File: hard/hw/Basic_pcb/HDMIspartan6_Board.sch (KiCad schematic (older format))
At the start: 50 parts

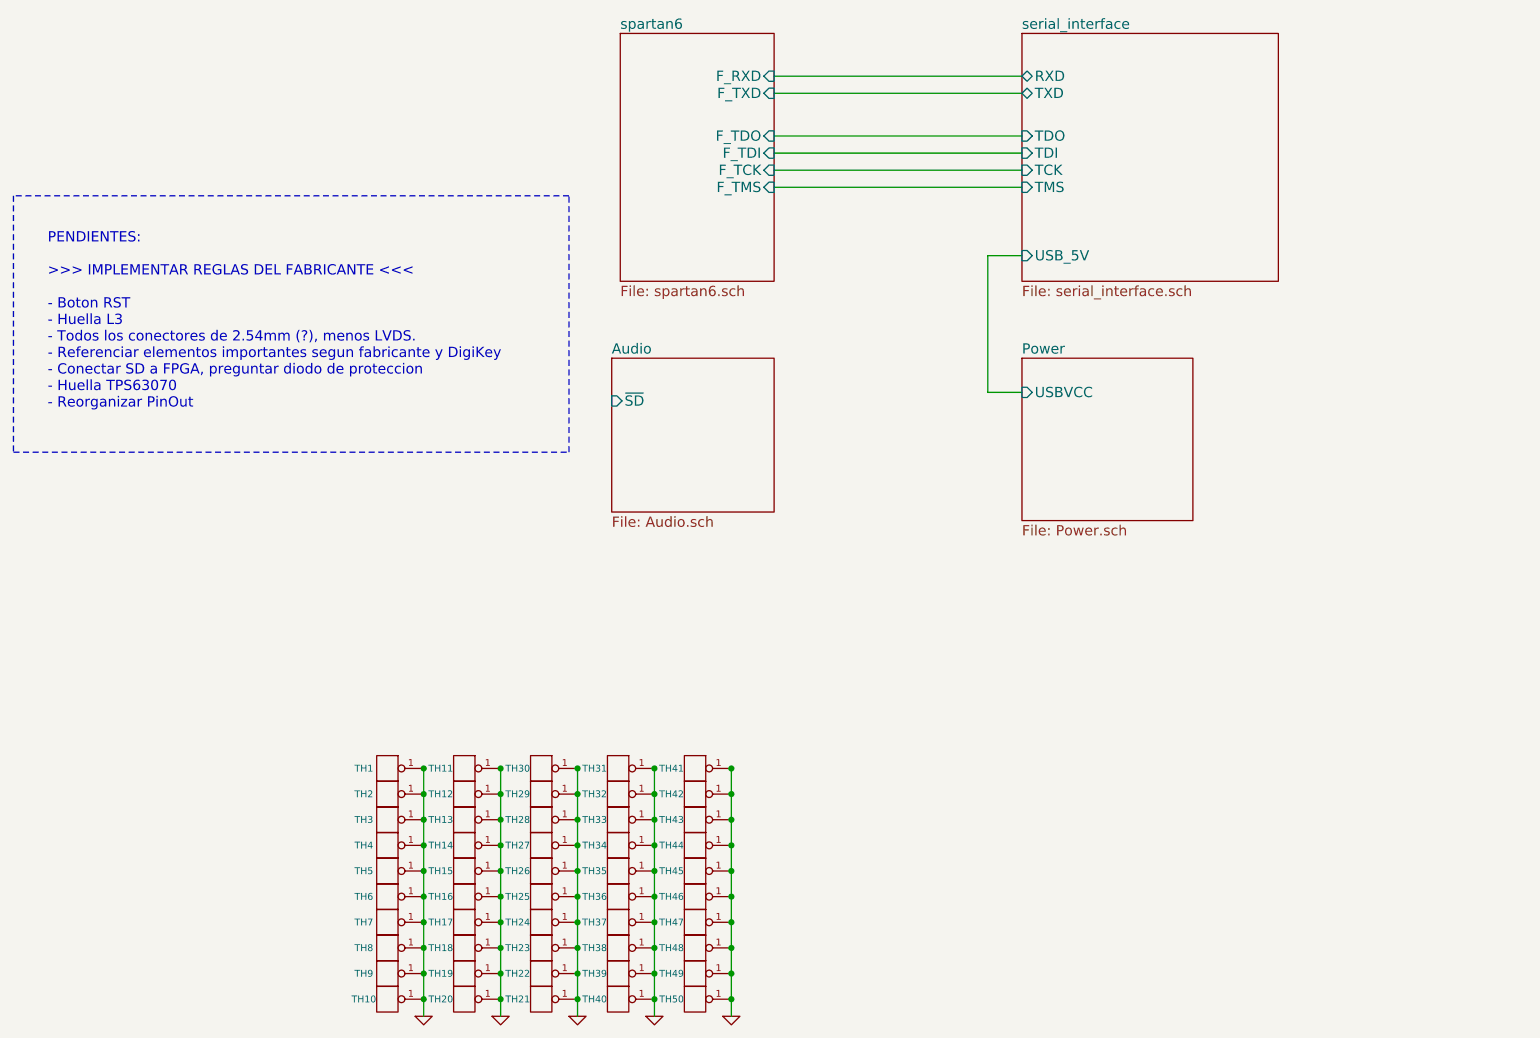
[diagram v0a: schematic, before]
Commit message: todas las huellas
by Ruben
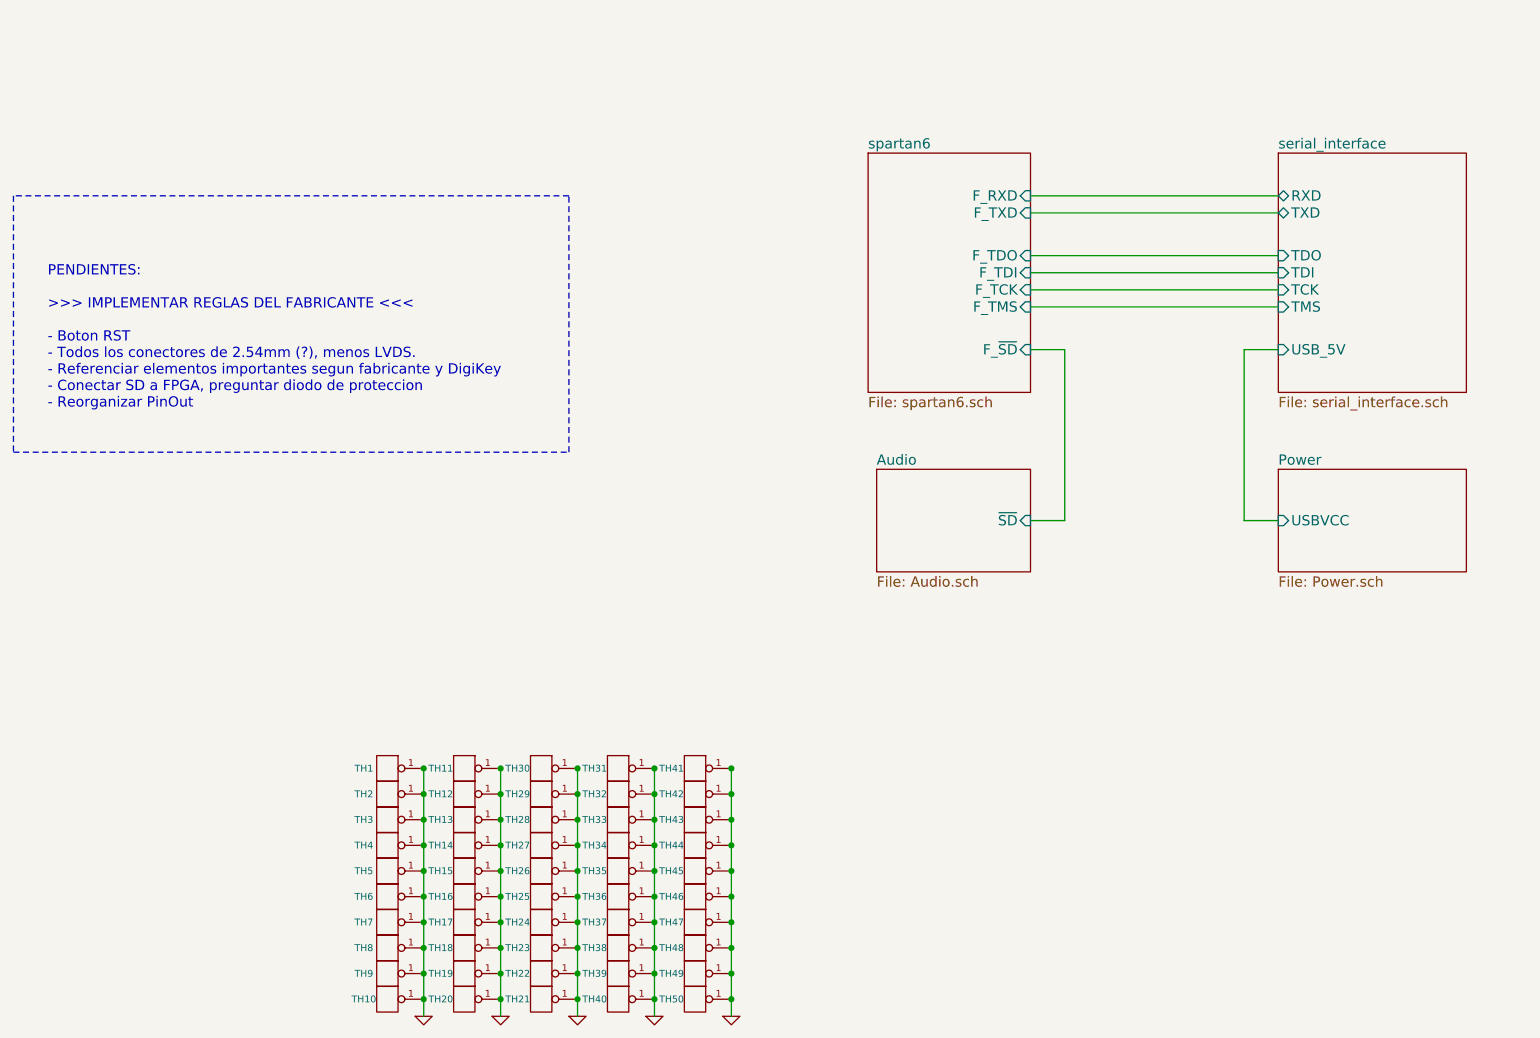
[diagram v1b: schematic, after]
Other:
- note added: "PENDIENTES:\n\n>>> IMPLEMENTAR REGLAS DEL FABRICANTE <<<\n\n- Boton RST\n- Todos los conectores de 2.54mm (?), menos LVDS.\n- Referenciar elementos importantes segun fabricante y DigiKey\n- Conectar SD a FPGA, preguntar diodo de proteccion\n- Reorganizar PinOut"
- note removed: "PENDIENTES:\n\n>>> IMPLEMENTAR REGLAS DEL FABRICANTE <<<\n\n- Boton RST\n- Huella L3\n- Todos los conectores de 2.54mm (?), menos LVDS.\n- Referenciar elementos importantes segun fabricante y DigiKey\n- Conectar SD a FPGA, preguntar diodo de proteccion\n- Huella TPS63070\n- Reorganizar PinOut"
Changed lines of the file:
@@
 $EndDescr
 $Sheet
-S 6650 1250 1500 1450
+S 8150 1950 1100 1400
 U 555AB8C7
 F0 "serial_interface" 60
 F1 "serial_interface.sch" 60
-F2 "TXD" B L 6650 1600 60
-F3 "RXD" B L 6650 1500 60
-F4 "TCK" I L 6650 2050 60
-F5 "TDI" I L 6650 1950 60
-F6 "TDO" I L 6650 1850 60
-F7 "TMS" I L 6650 2150 60
-F8 "USB_5V" I L 6650 2550 60
+F2 "TXD" B L 8150 2300 60
+F3 "RXD" B L 8150 2200 60
+F4 "TCK" I L 8150 2750 60
+F5 "TDI" I L 8150 2650 60
+F6 "TDO" I L 8150 2550 60
+F7 "TMS" I L 8150 2850 60
+F8 "USB_5V" I L 8150 3100 60
 $EndSheet
 $Comp
@@
 $EndComp
 $Sheet
-S 4250 3150 950  900
+S 5800 3800 900  600
 U 5898EE54
 F0 "Audio" 60
 F1 "Audio.sch" 60
-F2 "~SD" I L 4250 3400 60
+F2 "~SD" I R 6700 4100 60
 $EndSheet
 $Sheet
-S 4300 1250 900  1450
+S 5750 1950 950  1400
 U 54B6445D
 F0 "spartan6" 60
 F1 "spartan6.sch" 60
-F2 "F_TCK" I R 5200 2050 60
-F3 "F_TDI" I R 5200 1950 60
-F4 "F_TDO" I R 5200 1850 60
-F5 "F_TMS" I R 5200 2150 60
-F6 "F_RXD" I R 5200 1500 60
-F7 "F_TXD" I R 5200 1600 60
+F2 "F_TCK" I R 6700 2750 60
+F3 "F_TDI" I R 6700 2650 60
+F4 "F_TDO" I R 6700 2550 60
+F5 "F_TMS" I R 6700 2850 60
+F6 "F_RXD" I R 6700 2200 60
+F7 "F_TXD" I R 6700 2300 60
+F8 "F_~SD" I R 6700 3100 60
 $EndSheet
 $Sheet
-S 6650 3150 1000 950
+S 8150 3800 1100 600
 U 58991CBD
 F0 "Power" 60
 F1 "Power.sch" 60
-F2 "USBVCC" I L 6650 3350 60
+F2 "USBVCC" I L 8150 4100 60
 $EndSheet
 Wire Wire Line
-	6650 1850 5200 1850
-Wire Wire Line
-	6650 1950 5200 1950
-Wire Wire Line
-	6650 2050 5200 2050
-Wire Wire Line
-	6650 2150 5200 2150
-Wire Wire Line
-	5200 1500 6650 1500
-Wire Wire Line
-	6650 1600 5200 1600
-Wire Wire Line
-	6650 3350 6450 3350
-Wire Wire Line
-	6450 3350 6450 2550
-Wire Wire Line
-	6450 2550 6650 2550
+	8150 2550 6700 2550
+Wire Wire Line
+	8150 2650 6700 2650
+Wire Wire Line
+	8150 2750 6700 2750
+Wire Wire Line
+	8150 2850 6700 2850
+Wire Wire Line
+	6700 2200 8150 2200
+Wire Wire Line
+	8150 2300 6700 2300
 Text Notes 950  3450 0    60   ~ 0
-PENDIENTES:\n\n>>> IMPLEMENTAR REGLAS DEL FABRICANTE <<<\n\n- Boton RST\n- Huella L3\n- Todos los conectores de 2.54mm (?), menos LVDS.\n- Referenciar elementos importantes segun fabricante y DigiKey\n- Conectar SD a FPGA, preguntar diodo de proteccion\n- Huella TPS63070\n- Reorganizar PinOut
+PENDIENTES:\n\n>>> IMPLEMENTAR REGLAS DEL FABRICANTE <<<\n\n- Boton RST\n- Todos los conectores de 2.54mm (?), menos LVDS.\n- Referenciar elementos importantes segun fabricante y DigiKey\n- Conectar SD a FPGA, preguntar diodo de proteccion\n- Reorganizar PinOut
 Wire Notes Line
 	750  2200 750  3700
@@
 Wire Notes Line
 	4000 2200 750  2200
+Wire Wire Line
+	7950 4100 8150 4100
+Wire Wire Line
+	6700 3100 6900 3100
+Wire Wire Line
+	6900 3100 6900 4100
+Wire Wire Line
+	6900 4100 6700 4100
+Wire Wire Line
+	7950 4100 7950 3100
+Wire Wire Line
+	7950 3100 8150 3100
 $EndSCHEMATC
